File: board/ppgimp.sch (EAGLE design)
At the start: 26 parts, among them J1 VDD, J2 GND, J3 SPI, J4 I_Test, J5 R_test, J6 SDA, J7 SEL, U1 LM334Z/NOPB, U2 AD8400ARZ1, U3 AD8400ARZ10, U4 AD8400ARZ10, U5 AD5933YRSZ, U6 ADG1609

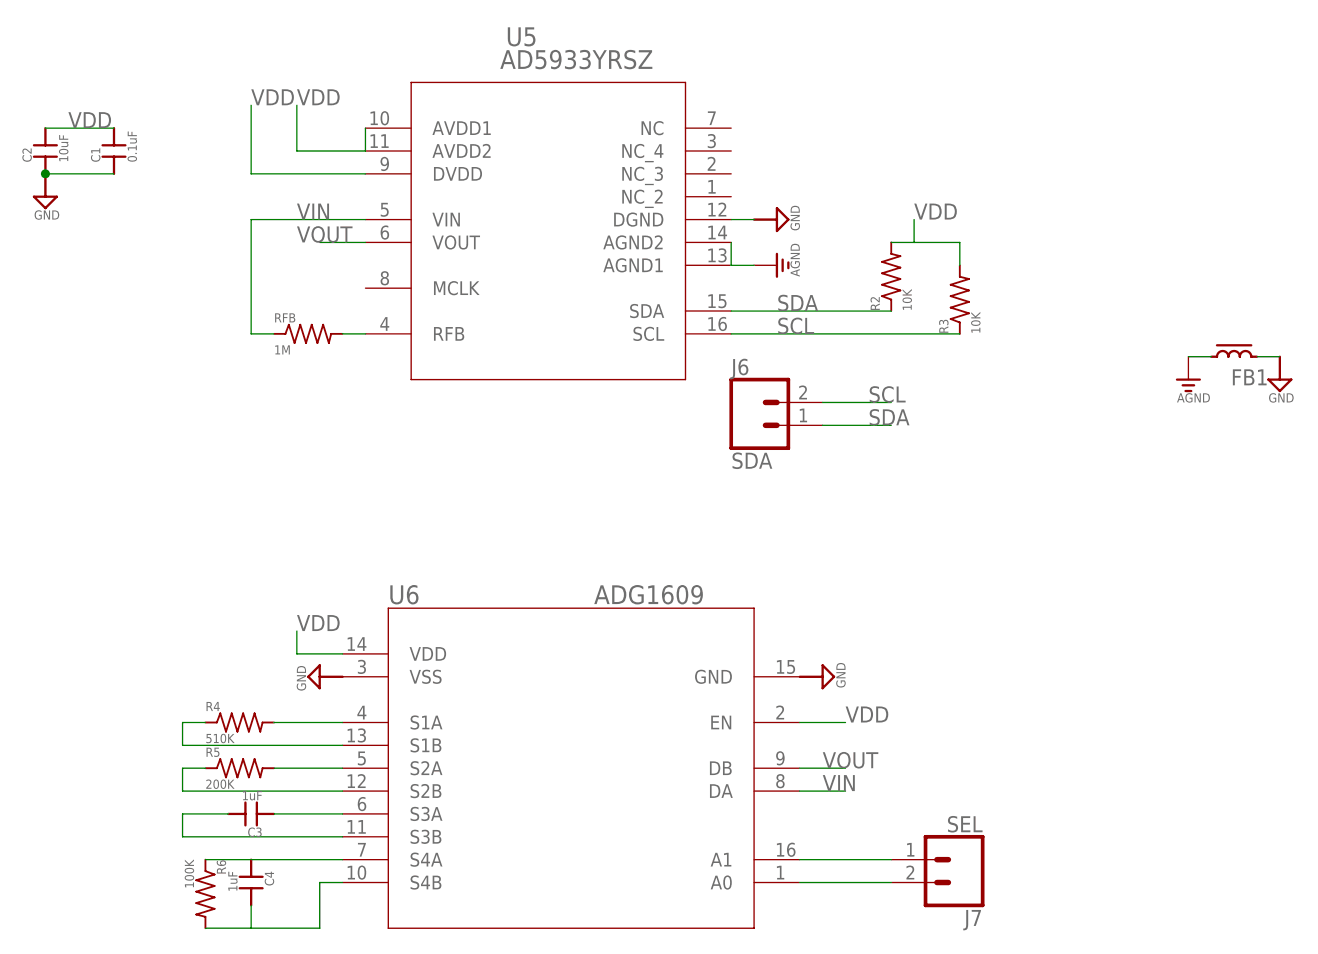
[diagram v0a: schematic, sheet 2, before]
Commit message: finalize prototype
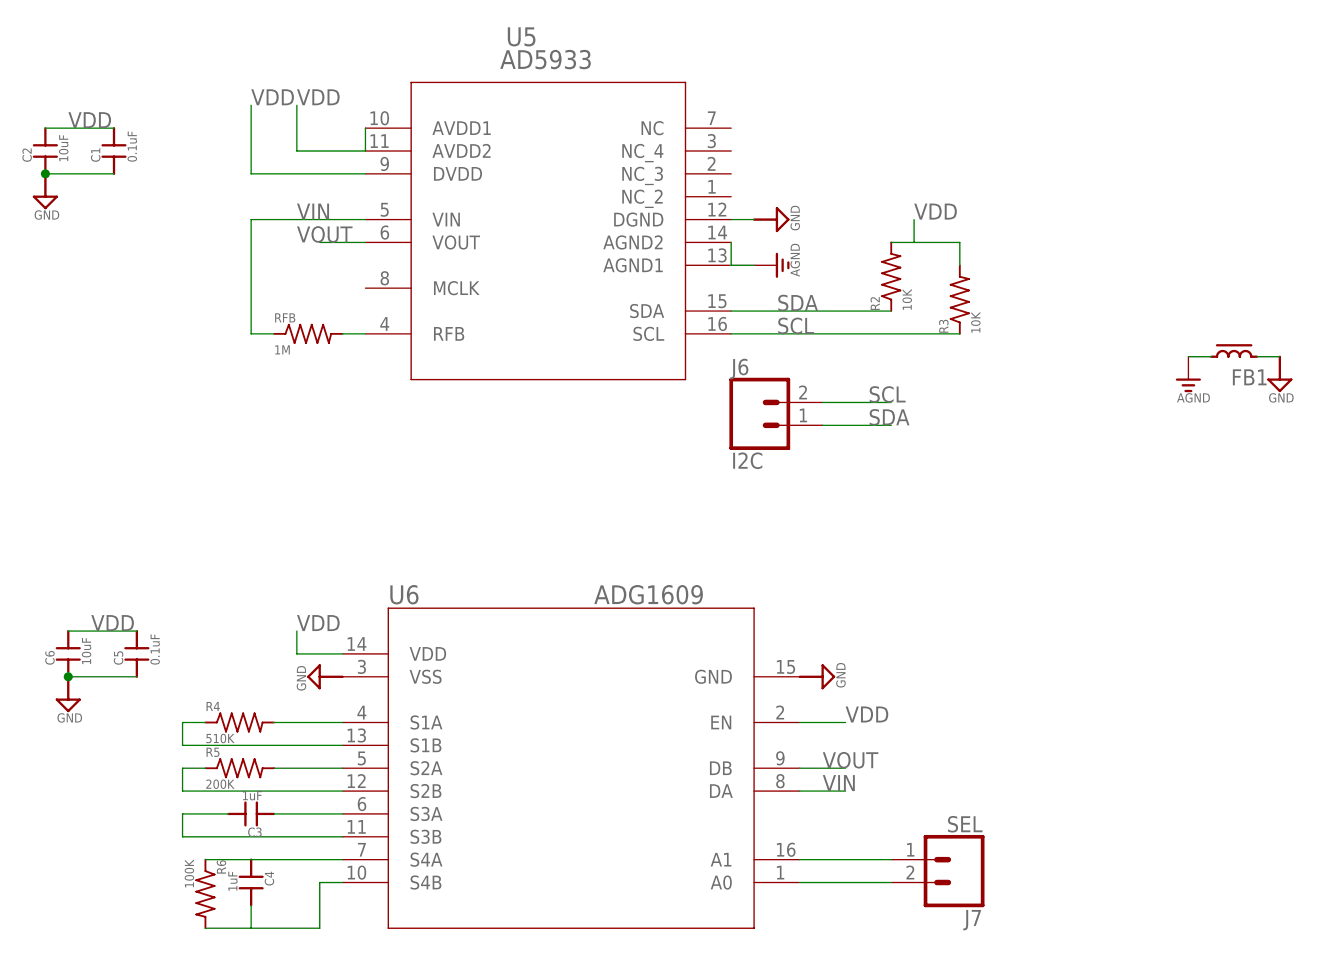
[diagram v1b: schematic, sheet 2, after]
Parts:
- added C5: 0.1uF, scono:CAP0603-CAP
- added C6: 10uF, scono:CAP0603-CAP
- J6: value SDA -> I2C
- U5: value AD5933YRSZ -> AD5933
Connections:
- net GND: now also C5.1, C6.1
- net VDD: now also C5.2, C6.2
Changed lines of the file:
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@@
 <attribute name="SUBSYSTEM_NAME" value="Imepdence"/>
 </part>
-<part name="U5" library="scono" deviceset="AD5933YRSZ" device=""/>
+<part name="U5" library="scono" deviceset="AD5933YRSZ" device="" value="AD5933"/>
 <part name="C1" library="scono" deviceset="CAP" device="0603-CAP" value="0.1uF"/>
 <part name="C2" library="scono" deviceset="CAP" device="0603-CAP" value="10uF"/>
@@
 <part name="SUPPLY7" library="scono" deviceset="AGND" device=""/>
 <part name="SUPPLY8" library="scono" deviceset="GND" device=""/>
-<part name="J6" library="scono" deviceset="CONN_02" device="" package3d_urn="urn:adsk.eagle:package:38039/1" value="SDA"/>
+<part name="J6" library="scono" deviceset="CONN_02" device="" package3d_urn="urn:adsk.eagle:package:38039/1" value="I2C"/>
 <part name="RFB" library="scono" deviceset="R-US_" device="R0603" value="1M"/>
 <part name="U6" library="scono" deviceset="ADG1609" device=""/>
@@
 <part name="R6" library="scono" deviceset="R-US_" device="R0603" value="100K"/>
 <part name="U1" library="scono" deviceset="LM334Z/NOPB" device=""/>
+<part name="C5" library="scono" deviceset="CAP" device="0603-CAP" value="0.1uF"/>
+<part name="C6" library="scono" deviceset="CAP" device="0603-CAP" value="10uF"/>
+<part name="SUPPLY13" library="scono" deviceset="GND" device=""/>
 </parts>
 <sheets>
@@
 <attribute name="VALUE" x="72.39" y="50.8" size="1.016" layer="96" rot="R270" align="top-left"/>
 </instance>
+<instance part="C5" gate="G$1" x="66.04" y="73.66" smashed="yes" rot="R90">
+<attribute name="NAME" x="64.516" y="72.39" size="1.016" layer="95" rot="R90"/>
+<attribute name="VALUE" x="68.58" y="72.39" size="1.016" layer="96" rot="R90"/>
+</instance>
+<instance part="C6" gate="G$1" x="58.42" y="73.66" smashed="yes" rot="R90">
+<attribute name="NAME" x="56.896" y="72.39" size="1.016" layer="95" rot="R90"/>
+<attribute name="VALUE" x="60.96" y="72.39" size="1.016" layer="96" rot="R90"/>
+</instance>
+<instance part="SUPPLY13" gate="GND" x="58.42" y="68.58" smashed="yes">
+<attribute name="VALUE" x="57.15" y="66.04" size="1.016" layer="96"/>
+</instance>
 </instances>
 <busses>
@@
 <label x="144.78" y="66.04" size="1.778" layer="95"/>
 </segment>
+<segment>
+<pinref part="C5" gate="G$1" pin="2"/>
+<pinref part="C6" gate="G$1" pin="2"/>
+<wire x1="66.04" y1="76.2" x2="58.42" y2="76.2" width="0.1524" layer="91"/>
+<label x="60.96" y="76.2" size="1.778" layer="95"/>
+</segment>
 </net>
 <net name="GND" class="0">
@@
 <pinref part="SUPPLY12" gate="GND" pin="GND"/>
 </segment>
-</net>
+<segment>
+<pinref part="C6" gate="G$1" pin="1"/>
+<pinref part="C5" gate="G$1" pin="1"/>
+<wire x1="58.42" y1="71.12" x2="66.04" y2="71.12" width="0.1524" layer="91"/>
+<pinref part="SUPPLY13" gate="GND" pin="GND"/>
+<junction x="58.42" y="71.12"/>
+</segment>
+</net>
